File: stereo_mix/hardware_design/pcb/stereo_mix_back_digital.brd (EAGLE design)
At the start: 70 x 100 mm, 194 parts, among them IC1 4051D, IC2 AMS1117-3.3, J1 WQP-PJ301M-12_JACK, J10 WQP-PJ301M-12_JACK, J11 WQP-PJ301M-12_JACK, J12 WQP-PJ301M-12_JACK, J13 WQP-PJ301M-12_JACK, J14 WQP-PJ301M-12_JACK, J15 WQP-PJ301M-12_JACK, J16 WQP-PJ301M-12_JACK, J17 CORTEX_DEBUG_PTH, J18 WQP-PJ301M-12_JACK, J19 WQP-PJ301M-12_JACK, J2 WQP-PJ301M-12_JACK, J3 WQP-PJ301M-12_JACK, J4 WQP-PJ301M-12_JACK, J5 WQP-PJ301M-12_JACK, J6 WQP-PJ301M-12_JACK, J7 WQP-PJ301M-12_JACK, J8 WQP-PJ301M-12_JACK, J9 WQP-PJ301M-12_JACK, U1 MCP4822E-SN, U10 MCP4822E-SN, U11 MCP6002T-I/SN, U12 MCP6002T-I/SN, U13 MCP4922E/SL, U14 MCP4922E/SL, U15 TL072CD, U16 TL072CD, U17 MCP6002T-I/SN, U18 MCP6002T-I/SN, U19 MCP6002T-I/SN, U2 MCP4822E-SN, U20 MCP6002T-I/SN, U21 STM32F030C8T6, U22 TL072CD, U3 MCP6002T-I/SN, U4 MCP6002T-I/SN, U5 MCP4922E/SL, U6 MCP4922E/SL, U7 TL072CD, U8 TL072CD, U9 MCP4822E-SN, X1 8MHz

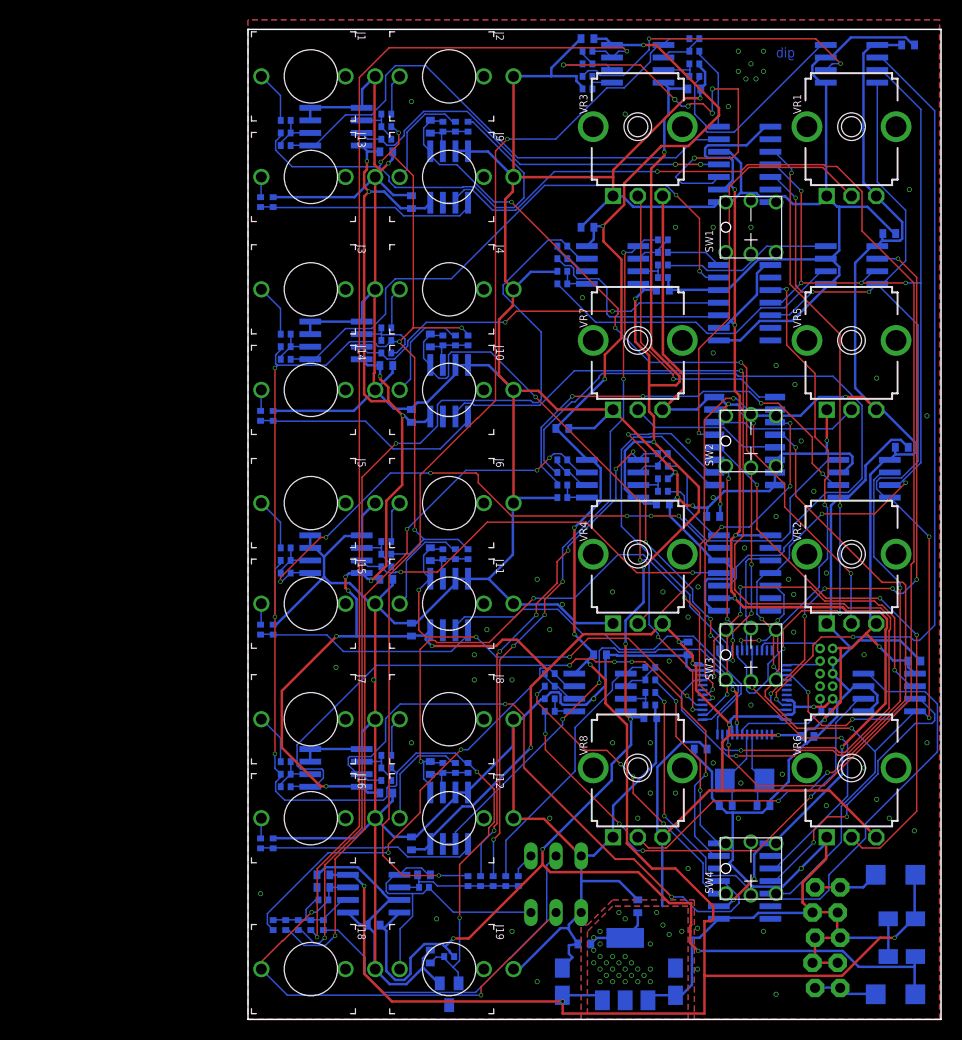
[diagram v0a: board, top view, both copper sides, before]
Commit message: stereo mix routing nearly finished
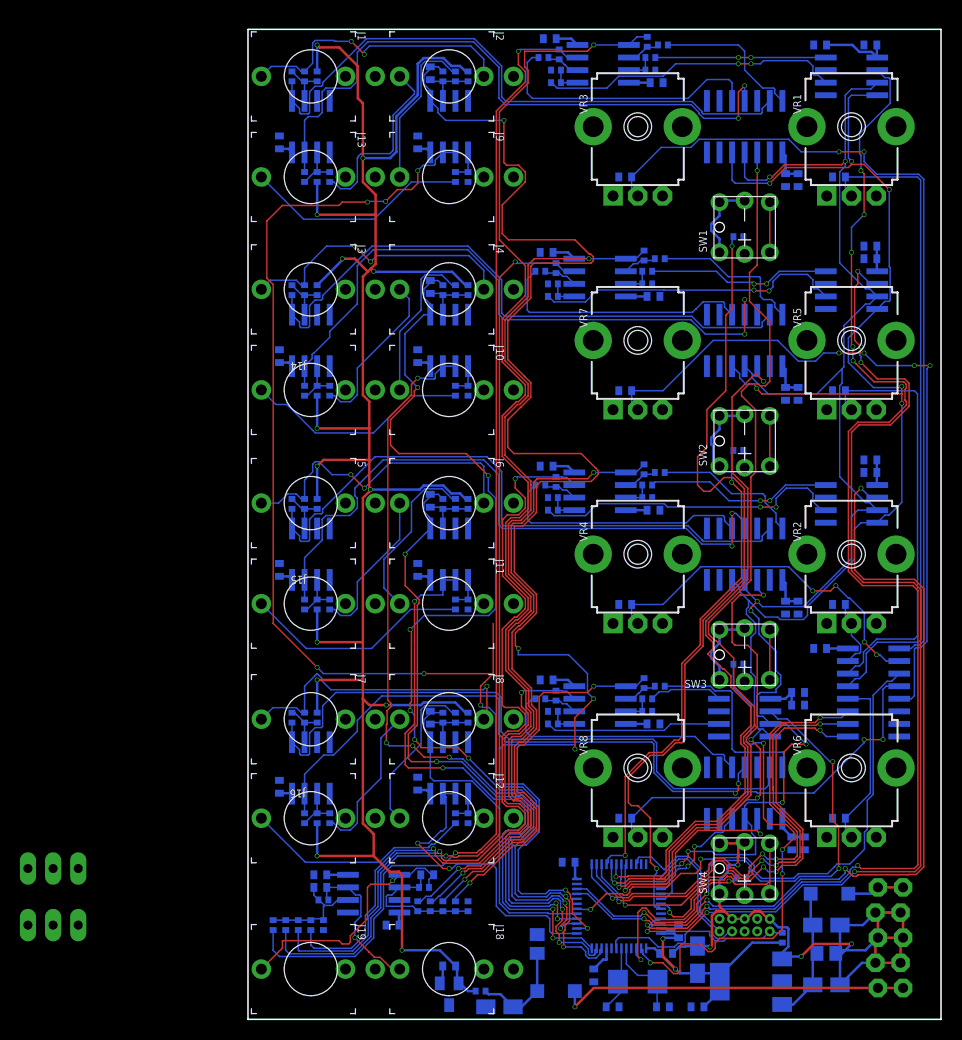
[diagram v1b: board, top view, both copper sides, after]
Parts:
- added C43, C44, C45, C46, C57, C58, C59, C60, C61, C62, C63, C64: 100nF, jhbruhn-cr:C0402
- added C47, C48: 22uF, jhbruhn-cdr:C0805
- added C49, C50, C51, C52, C53, C54, C55, C56: 10uF, jhbruhn-cr:C0402
- added R91, R92, R93, R94: 100R, jhbruhn-cdr:R0402
- C32, C33: value 6.8pF -> 220pF
- D1, D2: value SS54 -> B5819W; device jhbruhn-cdr:SMA -> jhbruhn-cdr:SOD123
- IC1: value 4051D -> 4051CD4051; device jhbruhn-ic:SO16 -> jhbruhn-ic:SOIC16N
- moved JP1 50.8 mm to (-19.7, 15.2)
- moved JP2 50.8 mm to (-19.7, 9.53)
- moved C38 41.0 mm to (25.4, 1.27)
- moved D2 34.3 mm to (31.1, 2.86), turned to 0 degrees
- moved C28 30.9 mm to (42.2, 6.67), turned to 180 degrees
- moved IC1 28.5 mm to (63.2, 33.0)
- moved C29 27.3 mm to (32.4, 15.9), turned to 0 degrees
- moved J17 26.7 mm to (50.2, 9.53), turned to 180 degrees
- moved C39 26.7 mm to (58.4, 3.49), turned to 0 degrees
- moved U21 25.0 mm to (37.5, 11.4)
- moved C27 23.3 mm to (36.8, 1.27), turned to 0 degrees
- moved R85 23.3 mm to (54.0, 8.26), turned to 270 degrees
- moved X1 23.0 mm to (39.4, 3.81)
- moved C26 22.7 mm to (41.9, 1.27)
- moved R81 19.8 mm to (22.2, 85.1), turned to 90 degrees
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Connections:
- removed net +5V: U13.1, U13.9, U14.1, U14.9, U5.1, U5.9, U6.1, U6.9
- new net LED_1: R91.1, U21.43
- new net LED_2: R92.1, U21.28
- new net LED_3: R93.1, U21.2
- new net LED_4: R94.1, U21.3
- new net N$12: R91.2, SW1.A
- new net N$13: R92.2, SW2.A
- new net N$18: R93.2, SW3.A
- new net N$42: R94.2, SW4.A
- new net SWITCH_1: SW1.1, SW1.2, U21.33
- new net SWITCH_2: SW2.1, SW2.2, U21.19
- new net SWITCH_3: SW3.1, SW3.2, U21.20
- new net SWITCH_4: SW4.1, SW4.2, U21.42
- net +12V: now also C48.1
- net +3V3: now also C43.1, C44.1, C45.1, C46.1, C49.1, C50.1, C51.1, C52.1, C53.1, C54.1, C55.1, C56.1, U13.1, U13.9, U14.1, U14.9, U5.1, U5.9, U6.1, U6.9
- net -12V: now also C47.2
- net 1_IN_L: now also J2.P$2_SWITCH
- net 2_IN_L: now also J4.P$2_SWITCH
- net 3_IN_L: now also J6.P$2_SWITCH
- net 4_IN_L: now also J8.P$2_SWITCH
- net GND: now also C43.2, C44.2, C45.2, C46.2, C47.1, C48.2, C49.2, C50.2, C51.2, C52.2, C53.2, C54.2, C55.2, C56.2, C57.2, C58.2, C59.2, C60.2, C61.2, C62.2, C63.2, C64.2, SW1.3, SW1.4, SW1.K, SW2.3, SW2.4, SW2.K, SW3.3, SW3.4, SW3.K, SW4.3, SW4.4, SW4.K
- net OUT_L: now also J18.P$2_SWITCH
- net PAN_1_POT: now also C61.1
- net PAN_2_POT: now also C62.1
- net PAN_3_POT: now also C63.1
- net PAN_4_POT: now also C64.1
- net VOL_1_POT: now also C57.1
- net VOL_2_POT: now also C58.1
- net VOL_3_POT: now also C59.1
- net VOL_4_POT: now also C60.1
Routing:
- net GND: track 835.6 -> 112.8 mm, vias 83 -> 4
- net +3V3: track 415.5 -> 75.2 mm, vias 52 -> 2
- net +12V: track 217.2 -> 25.4 mm, vias 9 -> 0
- net -12V: track 200.0 -> 20.2 mm, vias 9 -> 0
- net +5V: track 125.9 -> 0.00 mm, vias 7 -> 0
- net LED_1: track 0.00 -> 83.2 mm, vias 0 -> 2
- net PAN_CV_1: track 85.4 -> 157.9 mm
- net BIAS_DAC4_L: track 66.3 -> 7.52 mm, vias 2 -> 0
- net PAN_2_POT: track 15.5 -> 72.1 mm, vias 0 -> 4
- net PAN_1_POT: track 31.0 -> 84.9 mm, vias 1 -> 2
- net LED_3: track 0.00 -> 52.1 mm, vias 0 -> 4
- net LED_2: track 0.00 -> 49.7 mm, vias 0 -> 2
- net CS_BIAS_DAC_1: track 81.7 -> 130.0 mm, vias 2 -> 8
- net CS_BIAS_DAC_2: track 61.0 -> 108.9 mm
- net PAN_CV_2: track 60.2 -> 104.2 mm, vias 4 -> 8
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- removed copper zone on layer 1, net +3V3
- removed copper zone on layer 16, net +3V3
- removed copper zone on layer 1, net GND
- removed copper zone on layer 16, net GND
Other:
- board text removed: "gib"
